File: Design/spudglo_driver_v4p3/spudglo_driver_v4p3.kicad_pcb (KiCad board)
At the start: 4 copper layers, 70.2 x 40 mm, 99 parts, among them J1 locked, J2 Barrel_Jack_Switch, J4 Conn_01x08_Male, U1 receiver_433MHz, U10 STM32L431RCTx, U11 LP5907MFX-3.3, U12 USB-C-31-M-12, U13 XR21B1411, U14 NCP361, U2 TXS0104EDR, U3 receiver_433MHz, U4 receiver_433MHz, U5 receiver_433MHz, U6 PS2501-4, U7 ECS-.327-9-1210-TR, U8 ECS-480-8-36-RWN-TR, U9 SN74HCT245PW

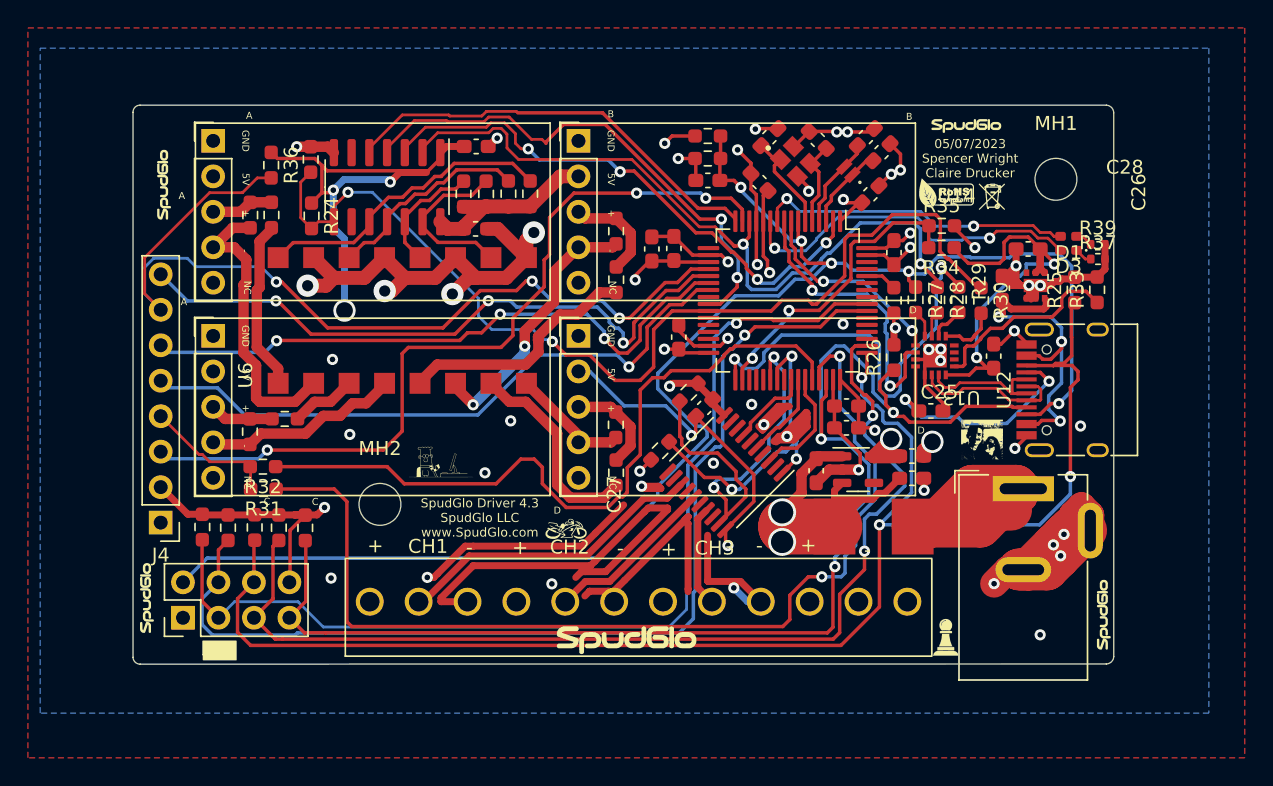
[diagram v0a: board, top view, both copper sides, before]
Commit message: spudglo v6 added
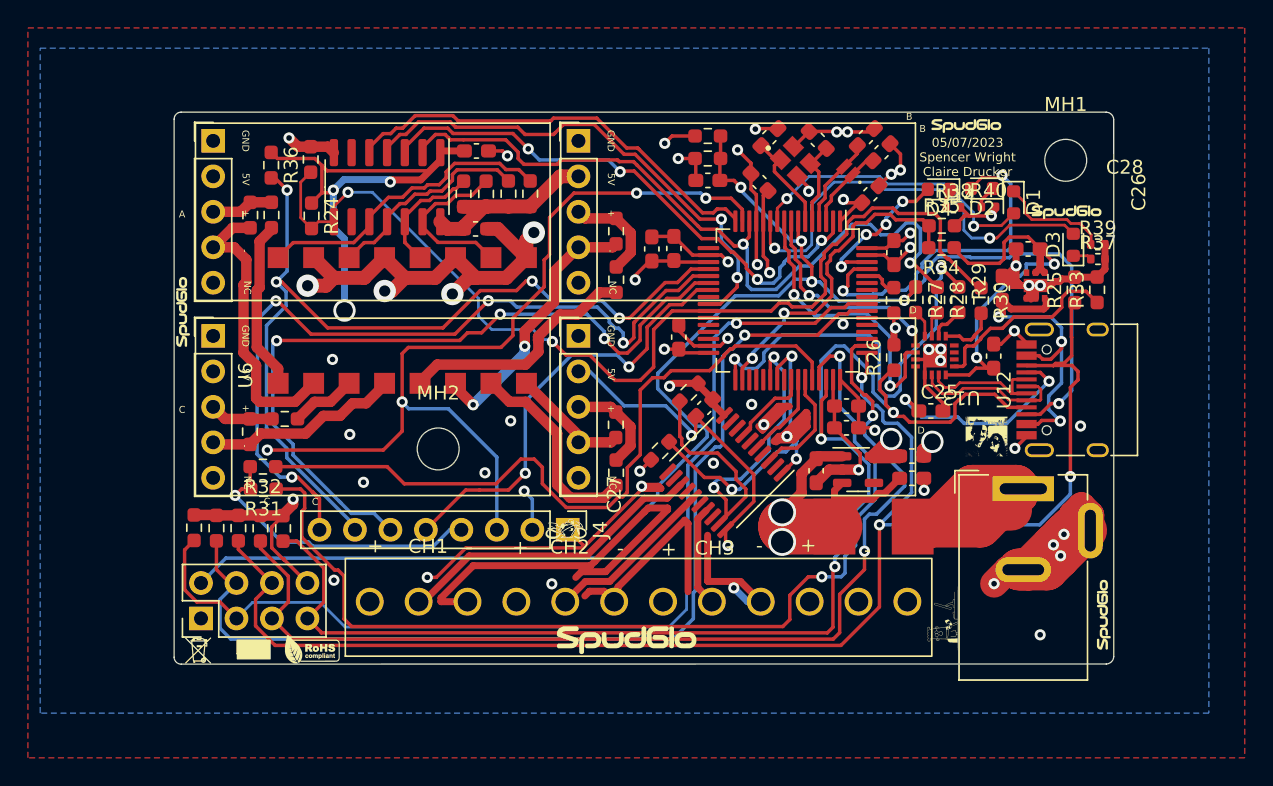
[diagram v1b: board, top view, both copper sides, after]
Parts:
- removed the G*** at (253.3, 85.6)
- added D2: BLUE LED, LED_SMD:LED_0603_1608Metric, F.Cu at (256.0, 53.5)
- added D4: ORANGE LED, LED_SMD:LED_0603_1608Metric, F.Cu at (252.9, 53.5)
- added R38: 100, Resistor_SMD:R_0402_1005Metric, F.Cu at (253.9, 54.8)
- added R40: 100, Resistor_SMD:R_0402_1005Metric, F.Cu at (256.4, 54.8)
- D1, D3: footprint LED_SMD:LED_0402_1005Metric_Pad0.77x0.64mm_HandSolder -> LED_SMD:LED_0603_1608Metric
- R37, R39: value 1k -> 100
- moved G*** 65.5 mm to (199.8, 86.5)
- moved G*** 64.7 mm to (262.0, 55.1), turned to 0 degrees
- moved G*** 55.9 mm to (208.0, 86.5)
- moved G*** 37.6 mm to (253.2, 84.2), turned to 90 degrees
- moved J4 29.2 mm to (226.3, 77.9), turned to -90 degrees
- moved G*** 20.6 mm to (198.8, 62.3)
- moved MH2 5.76 mm to (217.0, 72.1)
- moved D1 4.63 mm to (258.2, 54.4), turned to -90 degrees
- moved R18 1.59 mm to (205.9, 77.8)
- moved MH1 1.53 mm to (262.0, 51.4)
- moved R20 1.32 mm to (204.3, 77.8)
- moved J1 1.29 mm to (200.0, 84.2)
- moved R19 1.17 mm to (202.7, 77.8)
- moved R21 0.83 mm to (201.2, 77.8)
- moved R22 0.59 mm to (199.6, 77.7)
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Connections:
- U10 pad 61: unconnected-(U10-PB8/I2C1_SCL/TIM16_CH1-Pad61) -> /spudglo_v4p3_micro/BLUE_LED
- U10 pad 62: unconnected-(U10-PB9/I2C1_SDA/SPI2_NSS-Pad62) -> /spudglo_v4p3_micro/ORANGE_LED
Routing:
- net /spudglo_v4p3_micro/BLUE_LED: track 0.00 -> 24.9 mm, vias 0 -> 2
- net /spudglo_v4p3_micro/DISP_RST: track 45.5 -> 32.0 mm, vias 1 -> 2
- net Net-(J4-Pin_4): track 9.52 -> 21.1 mm, vias 0 -> 1
- net /spudglo_v4p3_micro/ORANGE_LED: track 0.00 -> 11.4 mm, vias 0 -> 4
- net /spudglo_v4p3_micro/DISP_BACKLIGHT: track 46.4 -> 57.6 mm, vias 3 -> 4
- net /spudglo_v4p3_micro/DISP_DC: track 44.7 -> 54.1 mm
- net Net-(D1-K): track 1.25 -> 7.96 mm
- net GND1: track 236.5 -> 243.0 mm, vias 51 -> 52
- net /spudglo_v4p3_micro/SPI1_SCK: track 57.7 -> 63.3 mm, vias 3 -> 4
- net /spudglo_v4p3_micro/RED_LED: track 25.6 -> 30.3 mm
- net /spudglo_v4p3_micro/SWDIO: track 95.0 -> 96.8 mm
- net Net-(D2-K): track 0.00 -> 1.66 mm
- net VBUS_PRESENT: track 22.1 -> 23.7 mm
- net Net-(D4-K): track 0.00 -> 1.39 mm
- net /spudglo_v4p3_micro/GREEN_LED: track 22.7 -> 21.3 mm
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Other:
- board size 70.2 x 40 mm -> 67.3 x 39.5 mm
